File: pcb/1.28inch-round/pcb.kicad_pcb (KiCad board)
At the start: 2 copper layers, 37.5 x 38.8 mm, 17 parts, among them J1 vik-module-connector, J2 vik-module-connector, J3 Conn_01x12_Pin, Q1 S8050

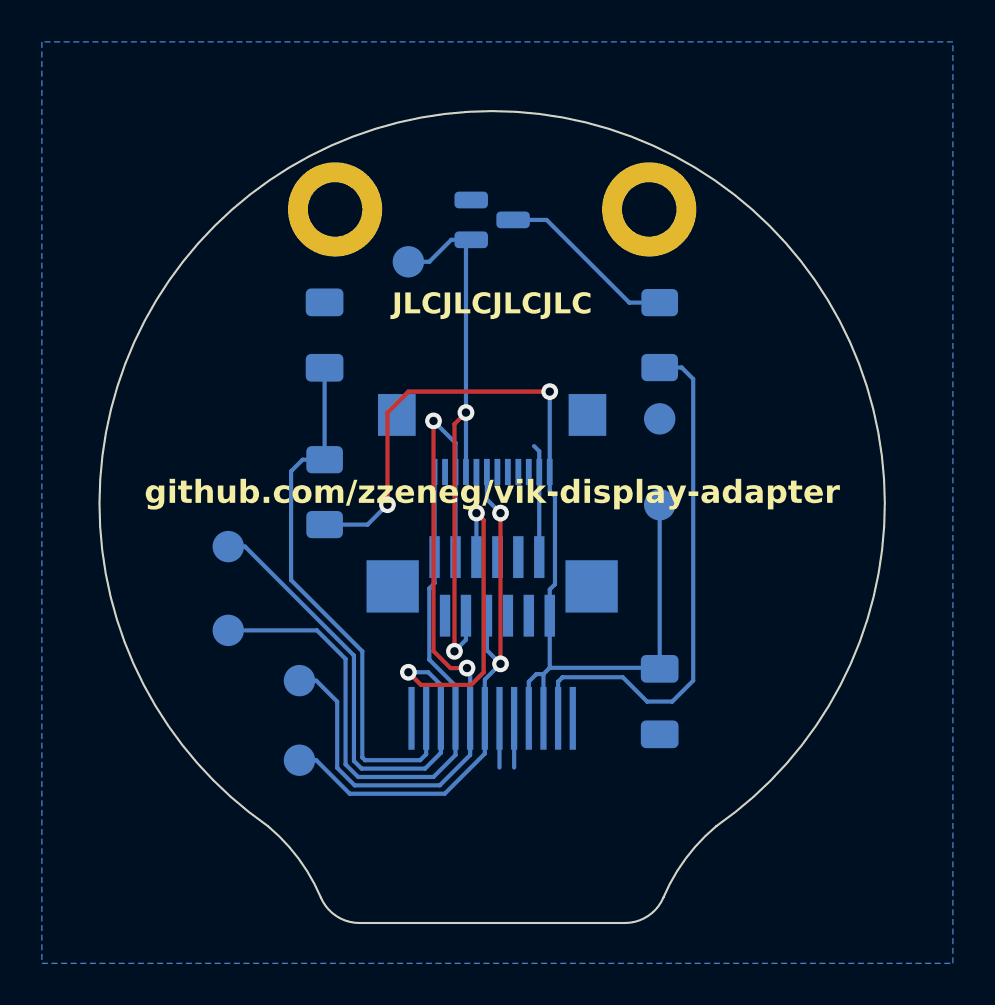
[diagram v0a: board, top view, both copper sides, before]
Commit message: small updates
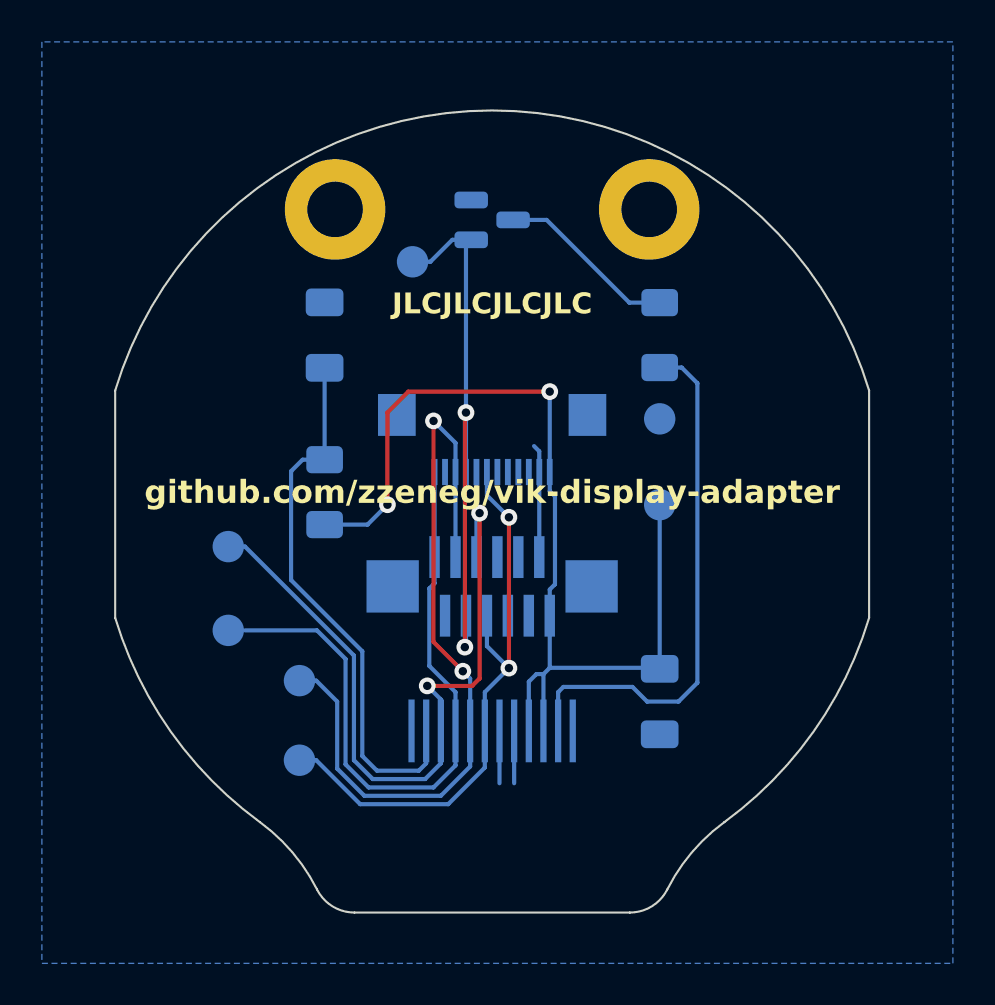
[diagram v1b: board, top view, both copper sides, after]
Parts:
- moved J3 0.60 mm to (99.5, 84.6)
- moved TP5 0.20 mm to (95.7, 62.2)
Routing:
- net MOSI: track 38.8 -> 36.7 mm
- net DC: track 27.2 -> 28.7 mm
- net GND: track 9.60 -> 11.1 mm
- net BLK: track 27.2 -> 26.1 mm
- net SCLK: track 30.5 -> 31.2 mm
- net RESET: track 26.2 -> 26.9 mm
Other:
- board size 37.5 x 38.8 mm -> 36 x 38.3 mm
- board text added: "v0.2"
- board text removed: "v0.1"
